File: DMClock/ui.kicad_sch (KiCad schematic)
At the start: 142 parts, among them U3 HV5622PG-G, U4 HV5622PG-G, U5 HV5622PG-G

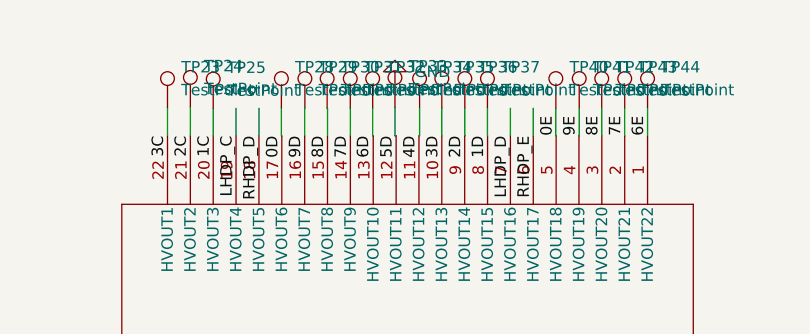
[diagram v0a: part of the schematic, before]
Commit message: finished v.1
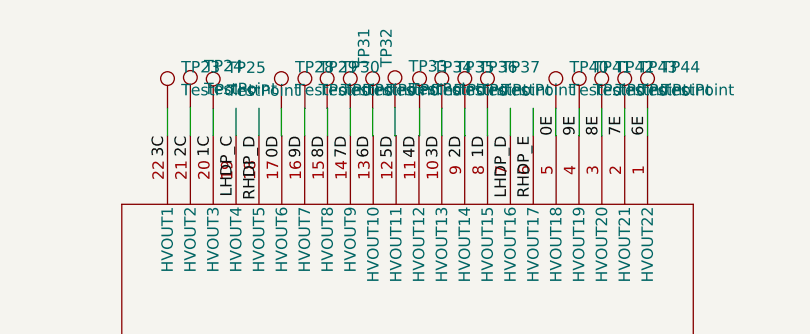
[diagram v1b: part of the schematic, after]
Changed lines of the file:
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@@
   )
   (symbol (lib_id "Connector:TestPoint") (at 223.6366 20.955 0) (unit 1)
-    (in_bom yes) (on_board yes) (dnp no) (fields_autoplaced)
-    (property "Reference" "TP31" (at 225.1606 16.383 0)
+    (in_bom yes) (on_board yes) (dnp no)
+    (property "Reference" "TP31" (at 225.1606 16.383 90)
       (effects (font (size 1.27 1.27)) (justify left))
     )
@@
     )
   )
-  (symbol (lib_id "power:GND") (at 228.6 18.161 180) (unit 1)
-    (in_bom yes) (on_board yes) (dnp no)
-    (property "Reference" "#PWR025" (at 228.6 11.811 0)
-      (effects (font (size 1.27 1.27)) hide)
-    )
-    (property "Value" "GND" (at 230.759 16.891 0)
-      (effects (font (size 1.27 1.27)) (justify right))
-    )
-    (property "Footprint" "" (at 228.6 18.161 0)
-      (effects (font (size 1.27 1.27)) hide)
-    )
-    (property "Datasheet" "" (at 228.6 18.161 0)
-      (effects (font (size 1.27 1.27)) hide)
-    )
-    (pin "1")
-    (instances
-      (project "DMClock"
-        (path "/b42b345f-a3f2-4eff-9109-2f4619119d33/6e102def-f8db-44ea-948b-b7115f90d225"
-          (reference "#PWR025") (unit 1)
-        )
-      )
-    )
-  )
   (symbol (lib_id "Connector:TestPoint") (at 142.1952 73.787 180) (unit 1)
     (in_bom yes) (on_board yes) (dnp no) (fields_autoplaced)
@@
   )
   (symbol (lib_id "Connector:TestPoint") (at 226.1225 20.955 0) (unit 1)
-    (in_bom yes) (on_board yes) (dnp no) (fields_autoplaced)
-    (property "Reference" "TP32" (at 227.6465 16.383 0)
-      (effects (font (size 1.27 1.27)) (justify left))
-    )
+    (in_bom yes) (on_board yes) (dnp no)
+    (property "Reference" "TP32" (at 227.6465 16.383 90)
+      (effects (font (size 1.27 1.27)) (justify left))
+    )
